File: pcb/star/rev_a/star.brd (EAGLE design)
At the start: 61.4 x 100 mm, 3 parts

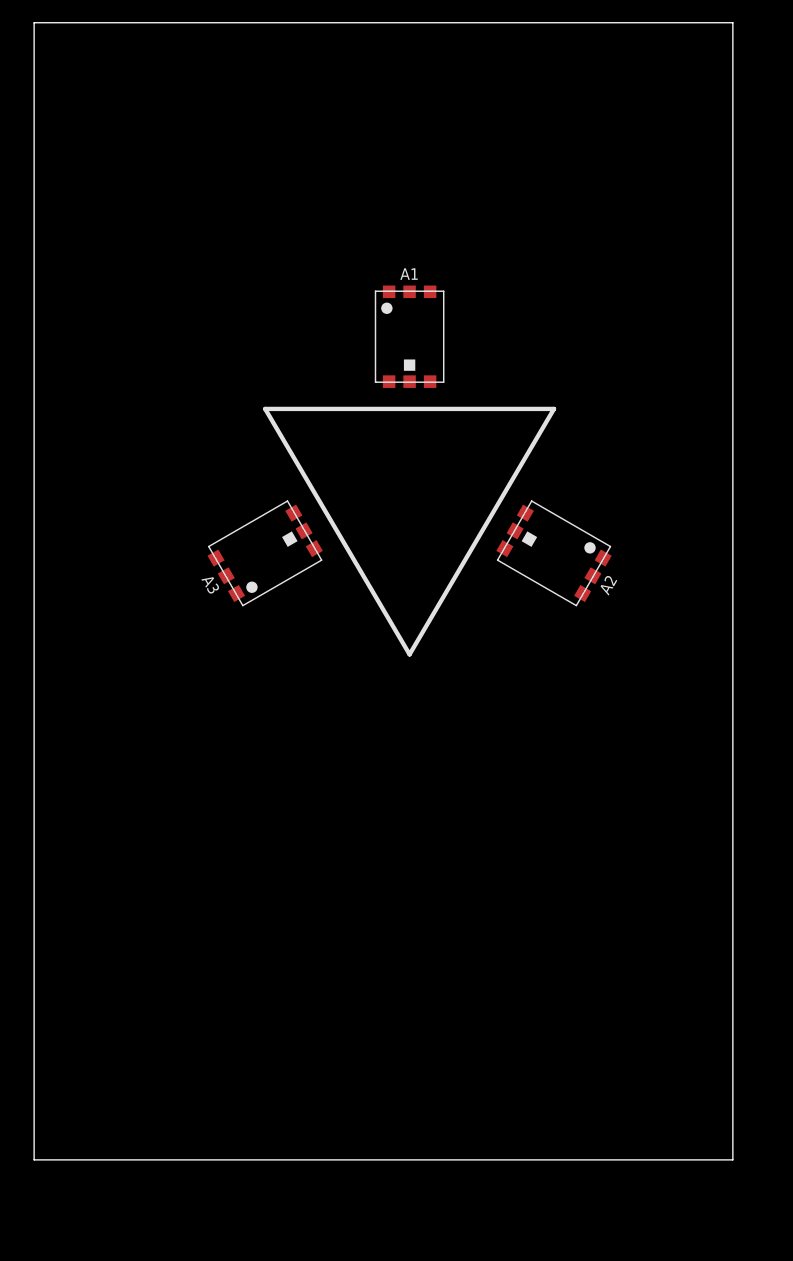
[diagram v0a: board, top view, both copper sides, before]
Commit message: got a shape
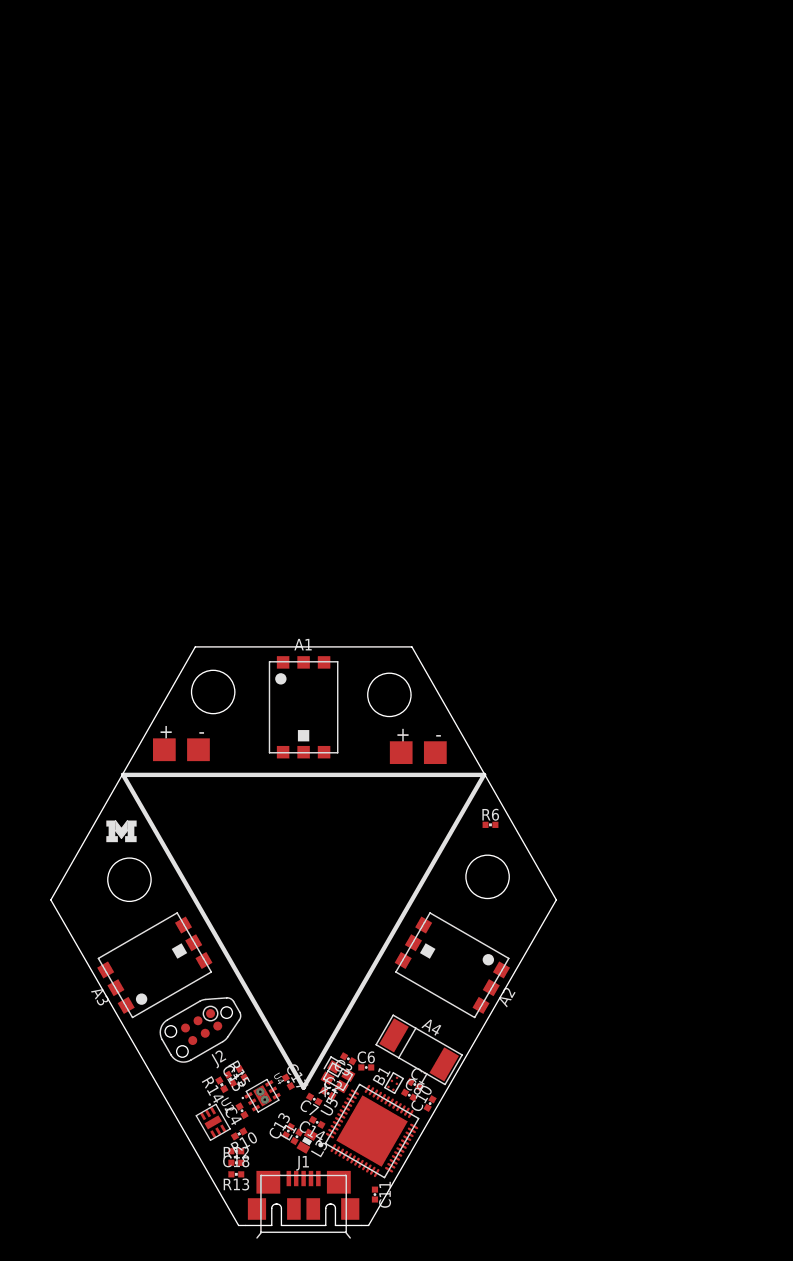
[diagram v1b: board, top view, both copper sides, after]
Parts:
- added A4: FRACTUS-2.4GHZ-FR05-S1-N-0-102, chips:FRACTUS-ANTENNA-FR05-S1-N-0-102
- added B1: BAL-NRF01D3, chips:BAL-NRF01D3
- added C1: 0.8pF, passives:0402_CAP
- added C10: 47nF, passives:0402_CAP
- added C11, C15, C4: 0.1uF, passives:0402_CAP
- added C13, C18: 1uF, passives:0402_CAP
- added C14: 4.7uF, passives:0402_CAP
- added C17: 0.47uF, passives:0402_CAP
- added C2, C3: 12pF, passives:0402_CAP
- added C6: 1nF, passives:0402_CAP
- added C7: 100nF, passives:0402_CAP
- added C8: 2.2nF, passives:0402_CAP
- added J1: MICRO_USB_B_HIROSE_ZX62R-B-5P, connector:USB_MICRO_B-HIROSE-ZX62R-B-5P
- added J2: TC2030-JLINK-NL, connector:TC2030-IDC-NL
- added L1: 15nH, passives:0402_CAP
- added L3: 10uH, passives:0603_CAP
- added LOGO1: UMICH_SOLID_SMALL, logos:UMICH_SOLID_75MIL
- added R10: 25.5k, passives:0402_RES
- added R12: 1M, passives:0402_RES
- added R13: 2M, passives:0402_RES
- added R14: 2.2M, passives:0402_RES
- added R15: 10M, passives:0402_RES
- added R6: 12k, passives:0402_RES
- added U$1, U$2: BAT_FLAT_PAD, connector:BATTERY_FLAT_PAD
- added U2: LTC4065, chips:DFN-6/2MM
- added U4: TPS715AXX, chips:WDFN-6
- added U5: NRF51822QF, chips:QFN-48-6MM
- added X1: EPSON-FA-128, crystals:FA-128
- moved A3 37.5 mm to (10.6, 17.1)
- moved A2 37.3 mm to (36.8, 17.1)
- moved A1 33.9 mm to (23.7, 39.8)
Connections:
- new net !CHRG: R12.1, R13.2, U2.2
- new net !FRAM_CS: U5.21
- new net !FRAM_HOLD: U5.20
- new net !FRAM_WP: U5.22
- new net !RTC_INT: U5.44
- new net AIN3: U5.6
- new net AIN4: U5.7
- new net AIN5: U5.8
- new net AIN6: U5.9
- new net AIN7: U5.10
- new net ANTENNA: A4.1, B1.SE, C1.1
- new net AVDD: C13.1, C6.1, L1.1, U5.35, U5.36
- new net BATIN: C15.2, R14.2, R15.1
- new net BOOTLOADER_CTRL: U5.19
- new net BOOTLOADER_RX: U5.17
- new net BOOTLOADER_TX: U5.18
- new net DCC: L3.2, U5.2
- new net GND: B1.GND, C1.2, C10.2, C11.2, C13.2, C14.2, C15.1, C17.2, C18.2, C2.2, C3.2, C4.2, C6.2, C7.2, C8.2, J1.5, J2.5, R10.1, R13.1, R14.1, R6.1, U$1.M, U$2.M, U2.1, U2.5, U2.7, U4.2, U4.3, U4.4, U4.5, U4.TP, U4.TP2, U4.TP3, U5.13, U5.33, U5.34, U5.GND, X1.2, X1.4
- new net I2C_SCL: U5.5
- new net I2C_SDA: U5.11
- new net LED_BLUE: U5.27
- new net LED_GREEN: U5.28
- new net LED_RED: U5.26
- new net N$10: C2.1, U5.38, X1.3
- new net N$13: R10.2, U2.6
- new net N$15: C10.1, U5.29
- new net N$17: C7.1, U5.39
- new net N$18: B1.ANT1, U5.31
- new net N$19: B1.ANT2, U5.32
- new net N$20: B1.VCC, C8.1, U5.30
- new net N$37: L1.2, L3.1
- new net N$9: C3.1, U5.37, X1.1
- new net P08: U5.14
- new net P09: U5.15
- new net P10: U5.16
- new net P17: U5.25
- new net P21: U5.40
- new net P22: U5.41
- new net P23: U5.42
- new net P24: U5.43
- new net RTC_CE: U5.47
- new net SPI_MISO: U5.48
- new net SPI_MOSI: U5.3
- new net SPI_SCK: U5.4
- new net SWDCLK: J2.4, R6.2, U5.24
- new net SWDIO/!RESET: J2.2, U5.23
- new net VBAT: C4.1, R15.2, U$1.P, U$2.P, U2.3, U4.1
- new net VCC: C11.1, C14.1, C17.1, J2.1, U4.6, U5.1, U5.12
- new net VUSB: C18.1, J1.1, R12.2, U2.4
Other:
- board size 61.4 x 100 mm -> 44.5 x 50.9 mm

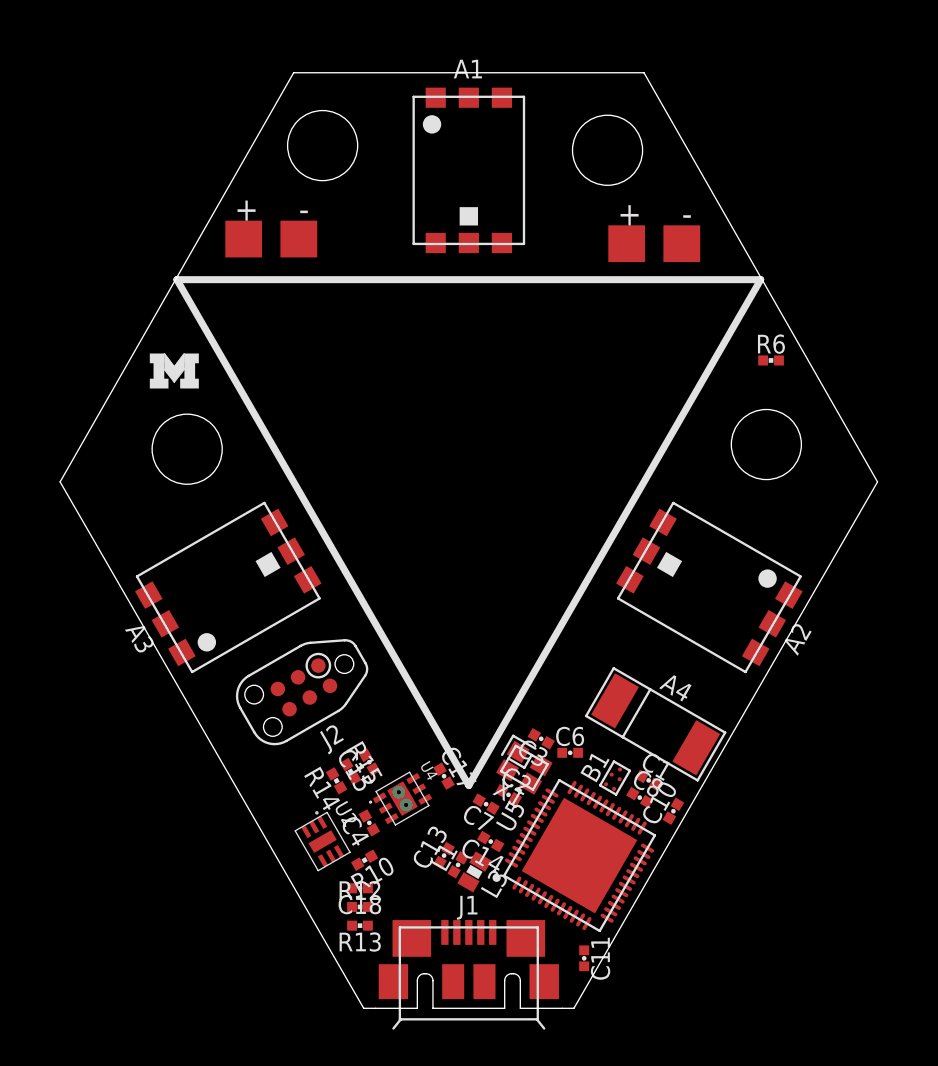
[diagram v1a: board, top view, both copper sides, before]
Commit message: new shape
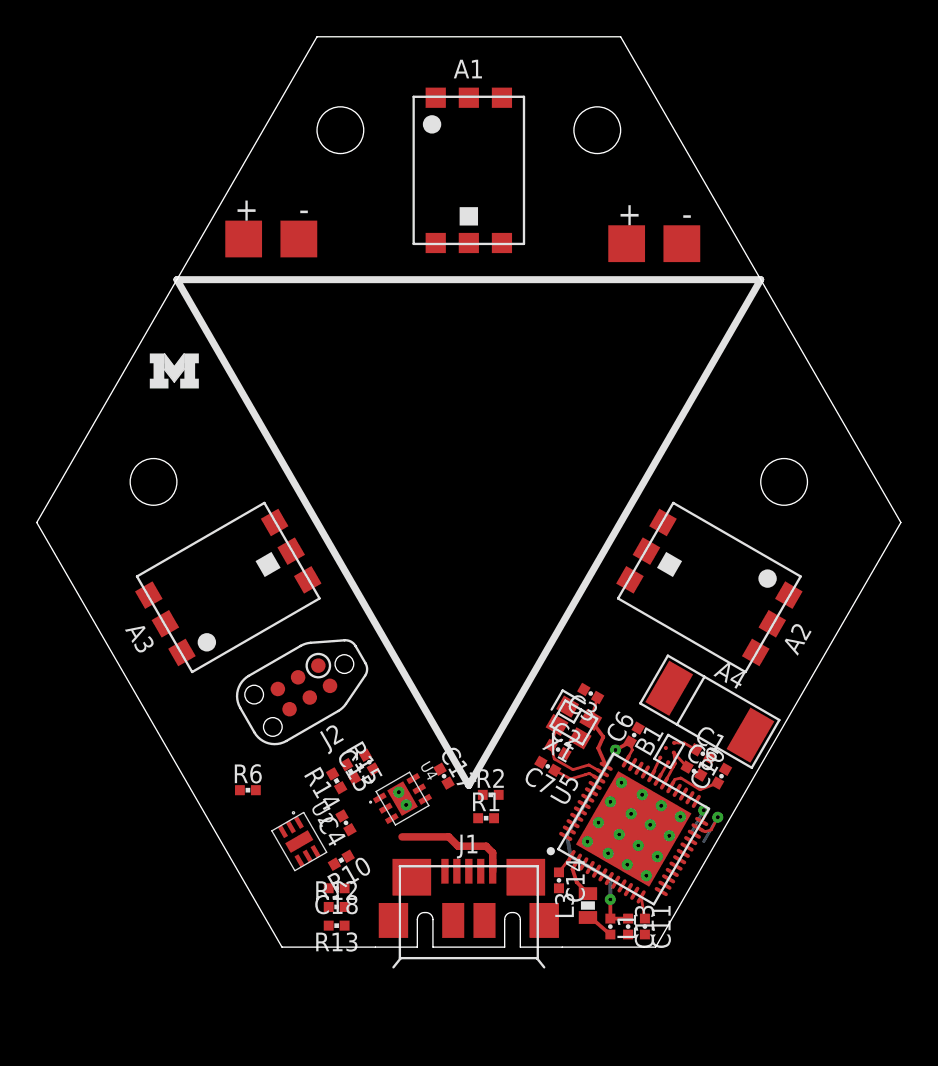
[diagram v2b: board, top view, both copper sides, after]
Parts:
- added R1, R2: 10k, passives:0402_RES
- moved R6 36.8 mm to (11.7, 6.10)
- moved C13 10.7 mm to (32.4, -1.32), turned to 270 degrees
- moved L1 8.93 mm to (31.4, -1.32), turned to 270 degrees
- moved L3 6.44 mm to (30.2, -0.18), turned to 90 degrees
- moved C14 4.27 mm to (28.6, 1.19), turned to 270 degrees
- moved C7 3.93 mm to (28.0, 7.39)
- moved C11 3.73 mm to (33.3, -1.32)
- moved C2 3.65 mm to (28.5, 8.31)
- moved X1 3.65 mm to (29.4, 9.78)
- moved C3 3.65 mm to (30.3, 11.4)
- moved C6 3.61 mm to (32.7, 9.09), turned to 60 degrees
- moved J1 3.33 mm to (23.7, -2.44)
- moved C8 3.28 mm to (35.9, 7.14)
- moved B1 3.28 mm to (34.6, 8.20)
- moved U5 3.28 mm to (32.7, 3.99)
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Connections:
- net !RTC_INT renamed DW_INT
- removed net !FRAM_CS: U5.21
- removed net !FRAM_HOLD: U5.20
- removed net !FRAM_WP: U5.22
- removed net AIN3: U5.6
- removed net AIN4: U5.7
- removed net AIN5: U5.8
- removed net AIN6: U5.9
- removed net AIN7: U5.10
- removed net BOOTLOADER_CTRL: U5.19
- removed net BOOTLOADER_RX: U5.17
- removed net BOOTLOADER_TX: U5.18
- removed net LED_BLUE: U5.27
- removed net LED_GREEN: U5.28
- removed net LED_RED: U5.26
- removed net P08: U5.14
- removed net P09: U5.15
- removed net P10: U5.16
- removed net P17: U5.25
- removed net P21: U5.40
- removed net P22: U5.41
- removed net P23: U5.42
- removed net P24: U5.43
- removed net RTC_CE: U5.47
- removed net SPI_MISO: U5.48
- removed net SPI_MOSI: U5.3
- removed net SPI_SCK: U5.4
- net I2C_SCL: now also R2.1, U5.47; no longer U5.5
- net I2C_SDA: now also R1.1, U5.48; no longer U5.11
- net VCC: now also R1.2, R2.2
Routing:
- net AVDD: track 0.00 -> 14.2 mm, vias 0 -> 2
- net VUSB: track 0.00 -> 6.29 mm
- net N$10: track 0.00 -> 4.84 mm
- net N$9: track 0.00 -> 4.18 mm
- net SWDIO/!RESET: track 0.00 -> 3.08 mm, vias 0 -> 1
- net N$15: track 0.00 -> 3.03 mm
- net N$20: track 0.00 -> 2.88 mm
- net N$17: track 0.00 -> 2.65 mm
- net VCC: track 0.00 -> 2.28 mm
- net DCC: track 0.00 -> 2.17 mm
- net SWDCLK: track 0.00 -> 2.03 mm, vias 0 -> 1
- net N$37: track 0.00 -> 1.59 mm
- net ANTENNA: track 0.00 -> 1.28 mm
- net N$19: track 0.00 -> 1.08 mm
- net N$18: track 0.00 -> 1.08 mm
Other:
- board size 44.5 x 50.9 mm -> 47 x 49.5 mm

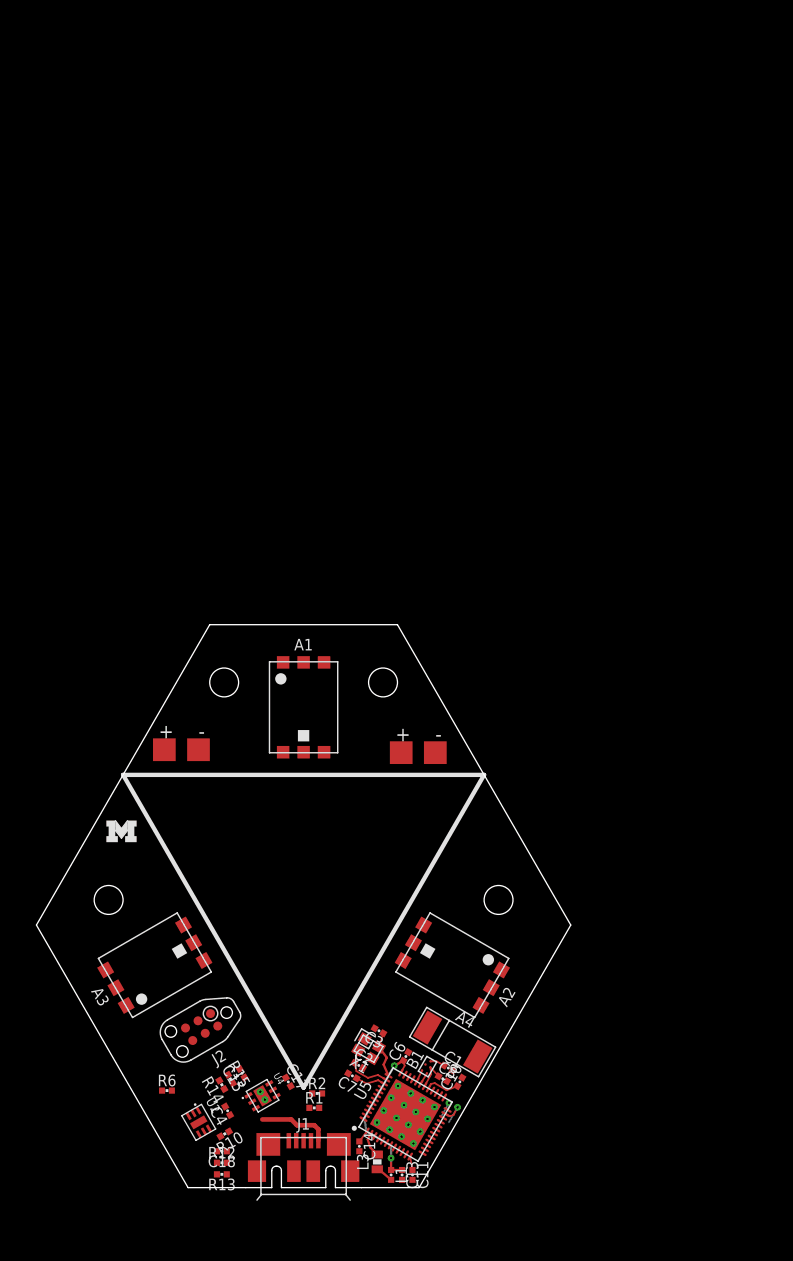
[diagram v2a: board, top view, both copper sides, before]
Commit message: more routing
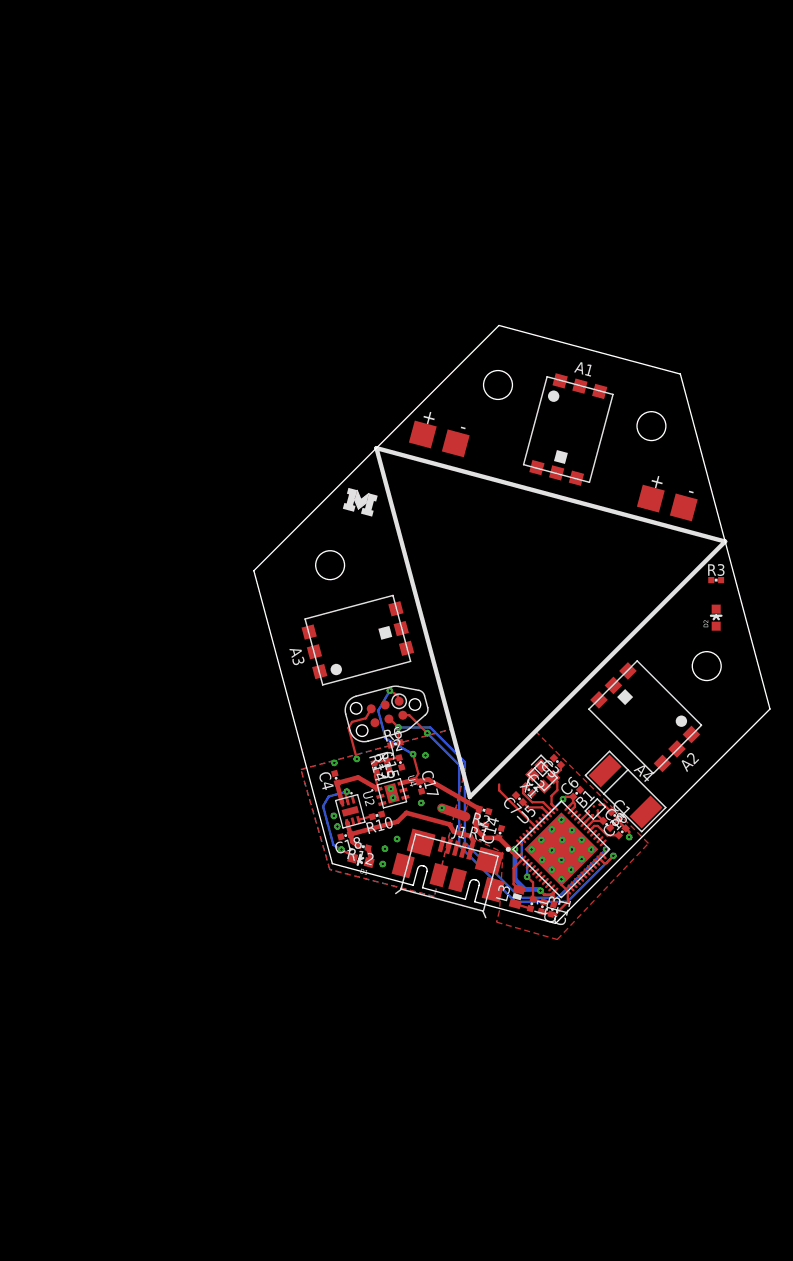
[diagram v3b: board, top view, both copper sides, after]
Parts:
- removed R13: 2M, passives:0402_RES
- added D1, D2: (no value), SparkFun-LED:LED-0603
- added R3: 1k, passives:0402_RES
- R10: value 25.5k -> 2k 1%
- R12: value 1M -> 1k
- moved R6 36.5 mm to (31.8, 36.6), turned to 15 degrees
- moved LOGO1 35.9 mm to (27.1, 57.3), turned to 345 degrees
- moved U$1 35.5 mm to (35.6, 63.4), turned to 345 degrees
- moved A1 33.7 mm to (47.0, 64.2), turned to 345 degrees
- moved A3 33.7 mm to (28.5, 45.7), turned to 105 degrees
- moved J2 32.1 mm to (31.0, 39.4), turned to 195 degrees
- moved R14 31.7 mm to (31.1, 34.7), turned to 105 degrees
- moved R10 31.0 mm to (30.2, 30.3), turned to 195 degrees
- moved U$2 31.0 mm to (55.7, 57.8), turned to 345 degrees
- moved C4 30.8 mm to (26.6, 33.6), turned to 105 degrees
- moved C15 30.7 mm to (32.2, 34.9), turned to 105 degrees
- moved R12 30.5 mm to (29.0, 27.5), turned to 165 degrees
- moved U2 30.4 mm to (27.8, 30.7), turned to 195 degrees
- moved C14 30.2 mm to (41.0, 28.7), turned to 75 degrees
- moved R15 30.2 mm to (30.0, 34.5), turned to 285 degrees
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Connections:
- new net !CHRG1: D2.A, R3.1
- new net N$5: D1.C, U2.2
- new net N$6: D2.C, U5.43
- net !CHRG: now also D1.A; no longer R13.2, U2.2
- net GND: no longer R13.1
- net VCC: now also R3.2
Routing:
- net SWDCLK: track 2.03 -> 33.6 mm, vias 1 -> 2
- net VCC: track 2.28 -> 33.7 mm, vias 0 -> 4
- net SWDIO/!RESET: track 3.08 -> 32.8 mm, vias 1 -> 2
- net GND: track 0.00 -> 16.0 mm, vias 16 -> 27
- net N$5: track 0.00 -> 9.19 mm, vias 0 -> 2
- net VUSB: track 6.29 -> 15.4 mm
- net VBAT: track 0.00 -> 7.30 mm
- net N$6: track 0.00 -> 5.06 mm
- net BATIN: track 0.00 -> 2.29 mm
- net !CHRG: track 0.00 -> 1.35 mm
- net N$13: track 0.00 -> 1.26 mm
- net DCC: track 2.17 -> 3.22 mm
- net AVDD: track 14.2 -> 14.7 mm
- added copper zone on layer 1, net GND
- added copper zone on layer 16, net GND
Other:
- board size 47 x 49.5 mm -> 45.4 x 52.6 mm

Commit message: update board
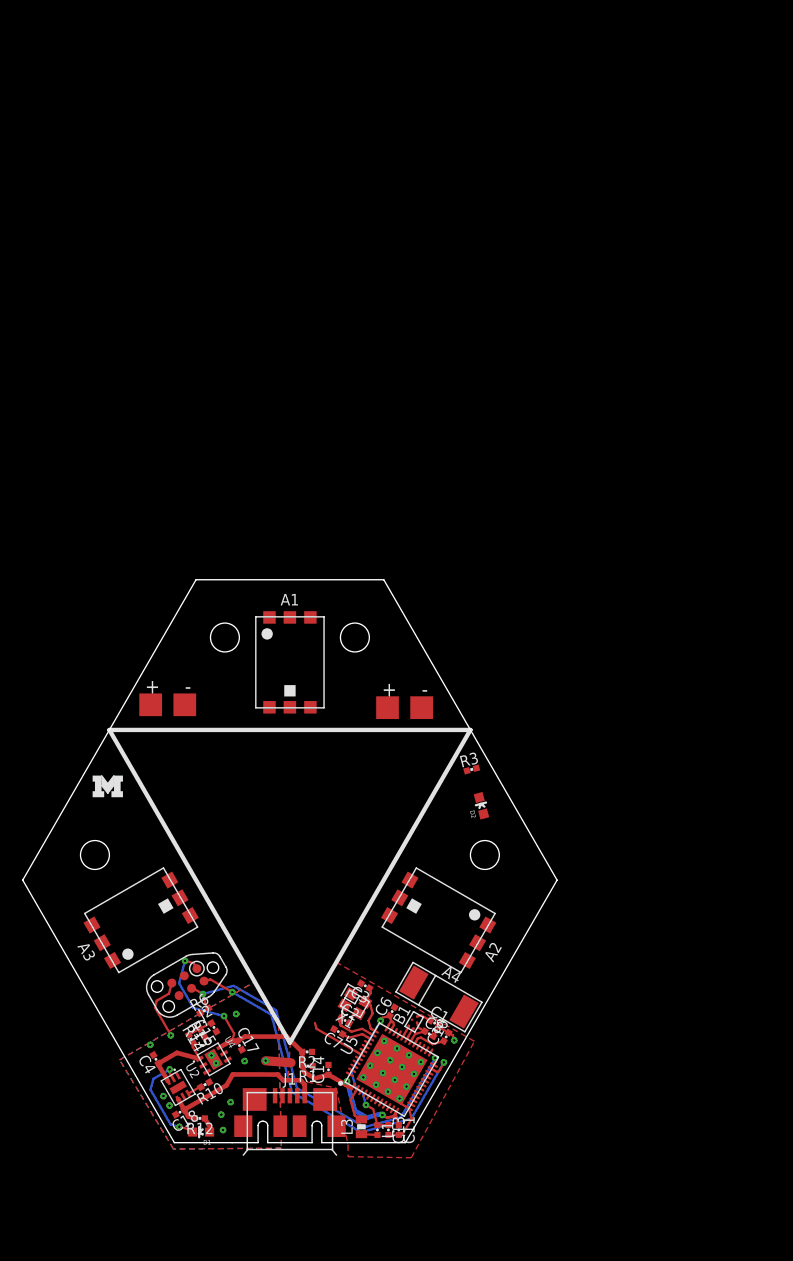
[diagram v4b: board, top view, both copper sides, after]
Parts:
- moved LOGO1 33.6 mm to (5.15, 31.9), turned to 0 degrees
- moved U$1 33.4 mm to (11.8, 40.0), turned to 0 degrees
- moved A1 31.9 mm to (22.5, 43.8), turned to 0 degrees
- moved A3 31.1 mm to (9.41, 21.1), turned to 120 degrees
- moved J2 29.5 mm to (13.5, 15.6), turned to 210 degrees
- moved C4 29.4 mm to (10.7, 8.85), turned to 120 degrees
- moved U$2 29.3 mm to (32.6, 39.8), turned to 0 degrees
- moved R6 28.9 mm to (15.0, 13.1), turned to 30 degrees
- moved R15 28.8 mm to (13.8, 10.6), turned to 300 degrees
- moved R14 28.7 mm to (14.8, 11.1), turned to 120 degrees
- moved U2 28.6 mm to (12.7, 6.37), turned to 210 degrees
- moved C15 28.5 mm to (15.8, 11.6), turned to 120 degrees
- moved C18 28.4 mm to (12.8, 4.20), turned to 210 degrees
- moved U4 28.2 mm to (15.8, 8.84), turned to 300 degrees
- moved R10 28.1 mm to (15.0, 6.62), turned to 210 degrees
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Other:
- board size 45.4 x 52.6 mm -> 47 x 49.5 mm
